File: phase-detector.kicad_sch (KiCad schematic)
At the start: 47 parts, among them J1 Conn_Coaxial_Small, J2 Conn_Coaxial_Small, J3 Conn_Coaxial_Small, J4 Conn_Coaxial_Small, J5 Conn_Coaxial_Small, J6 Conn_Coaxial_Small, J7 Conn_01x14_Socket, U14 LSM303C, U2 MIC5219-3.3YM5, U3 MIC5219-3.3YM5

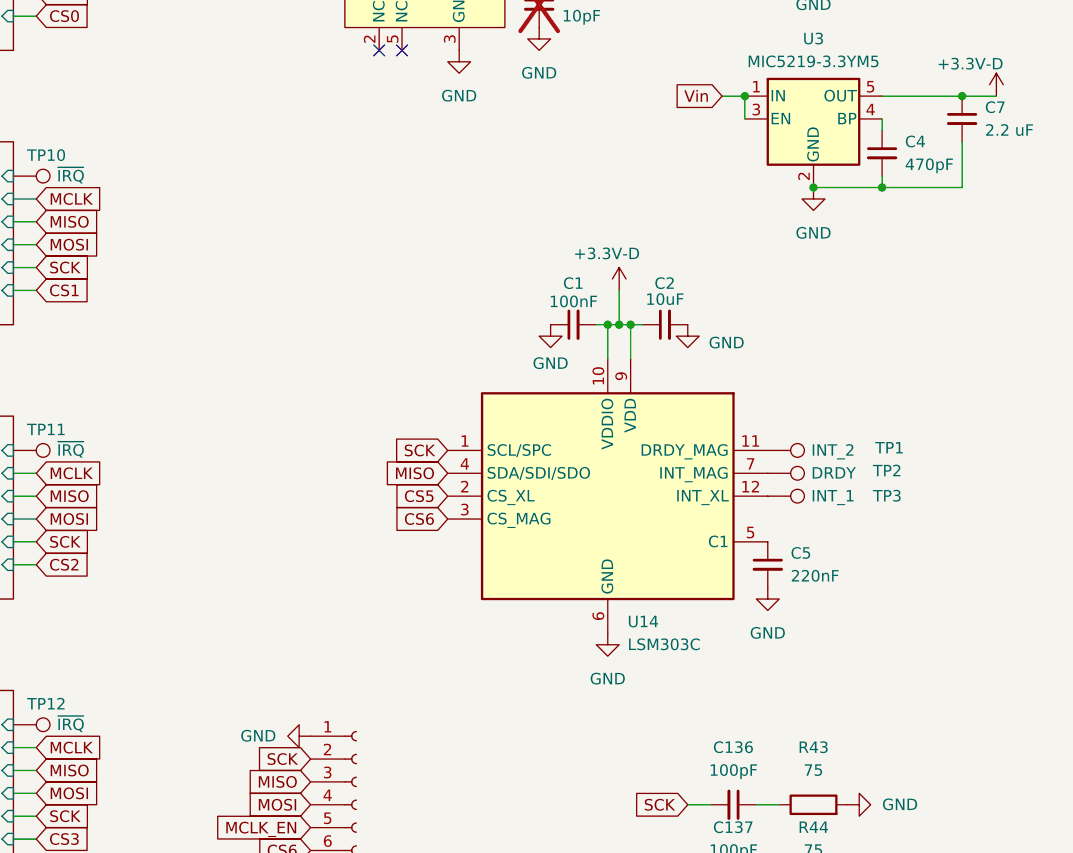
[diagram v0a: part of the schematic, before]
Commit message: boards ordered
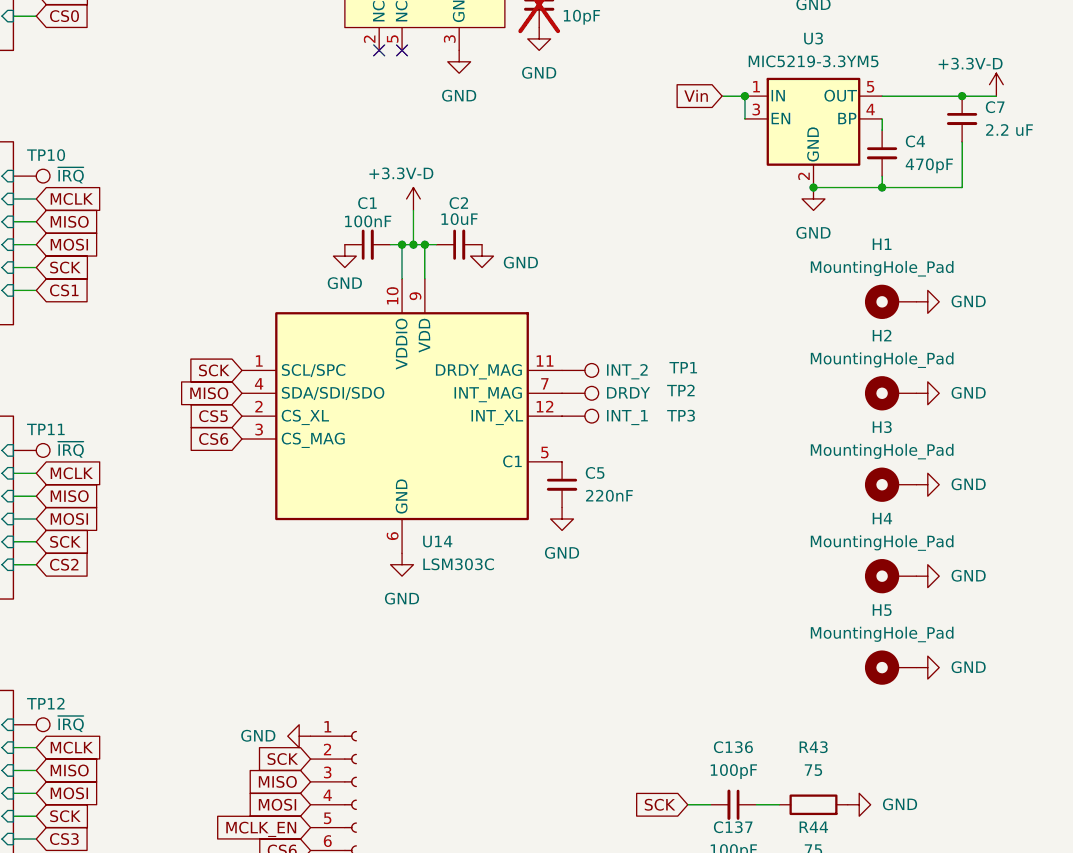
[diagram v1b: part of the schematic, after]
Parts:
- added H1, H2, H3, H4, H5: MountingHole_Pad, MountingHole:MountingHole_3.2mm_M3_Pad_TopBottom, symbol Mechanical:MountingHole_Pad
- J1, J2, J3, J4, J5: footprint Connector_Coaxial:SMA_Amphenol_132289_EdgeMount -> phase-detector:SMA_Amphenol_132289_EdgeMount
- J6: footprint Connector_Coaxial:SMA_Amphenol_132291-12_Vertical -> Connector_Coaxial:SMA_Amphenol_132134_Vertical
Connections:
- net GND: now also H1.1, H2.1, H3.1, H4.1, H5.1
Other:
- moved on the sheet: C1, C2, C5, TP1, TP2, TP3, U14
